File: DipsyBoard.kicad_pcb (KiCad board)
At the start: 2 copper layers, 22.9 x 50.8 mm, 31 parts, among them CON1 SDMMC_Card, P1 USB_OTG, P2 CONN_01X19, P3 CONN_01X19, P6 JTAG, SW1 SW_PUSH, U1 STM32L486Rx-LQFP64, U3 TPS56x200, U4 PUSBMxX4, X1 XTAL

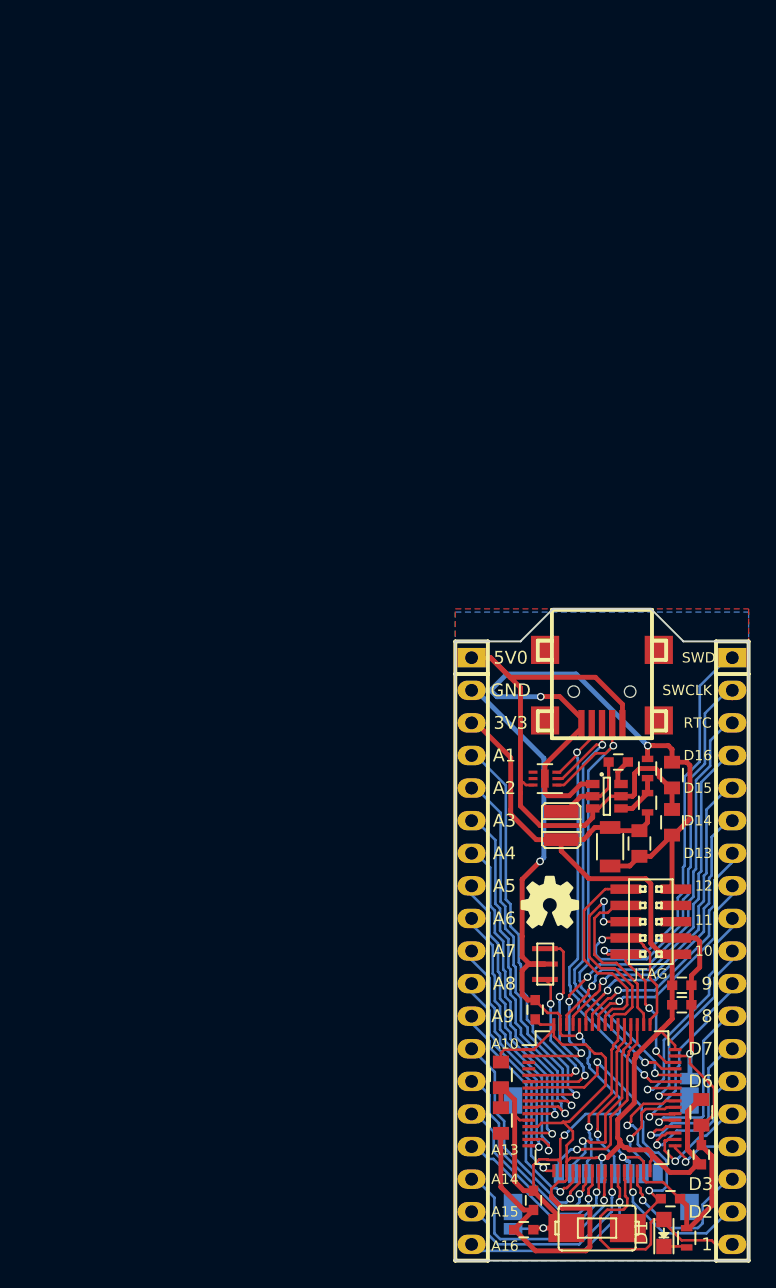
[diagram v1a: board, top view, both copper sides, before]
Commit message: v0.2
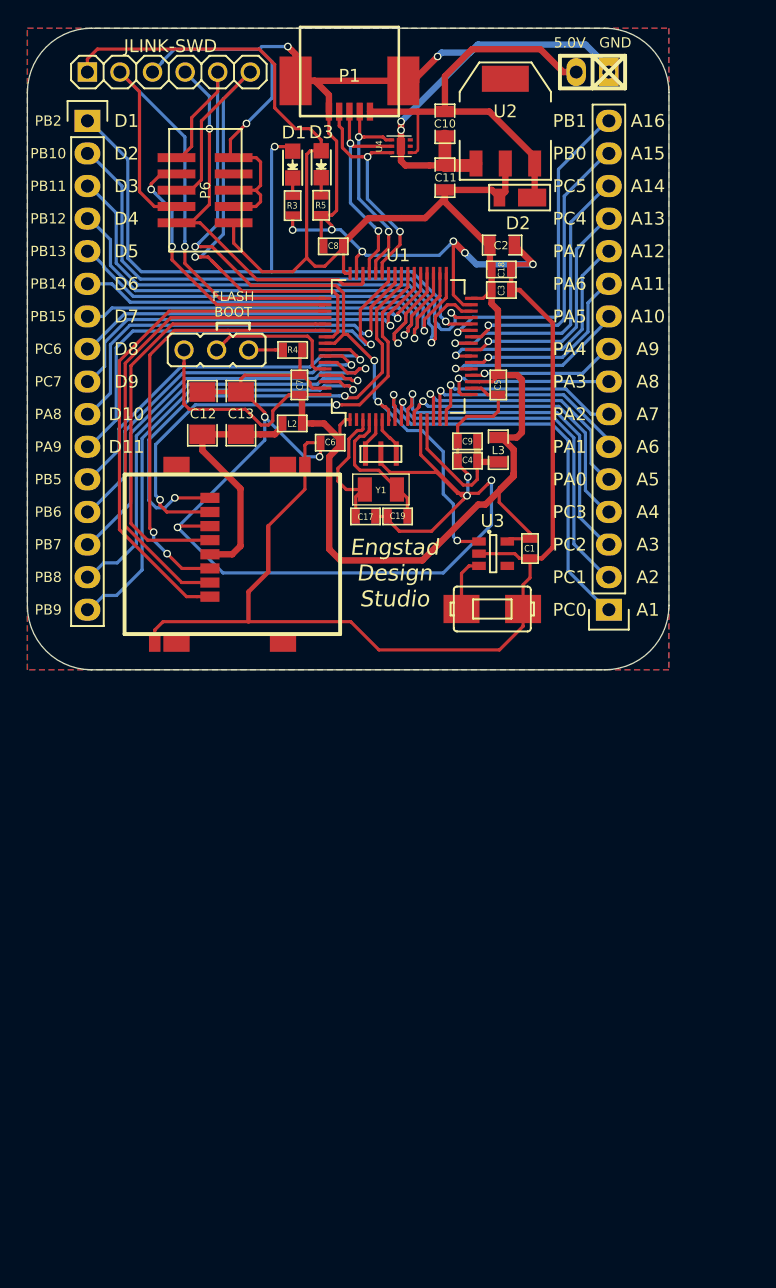
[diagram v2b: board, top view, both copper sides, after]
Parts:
- removed ?: , xess:oshw-logo2
- removed C14: 0.1uF, Capacitors_SMD:C_0603
- removed C15: 10uF, Capacitors_SMD:C_0805
- removed C16: 22uF, Capacitors_SMD:C_1206
- removed L1: 3.3uH, engstad:inductor-smd-1212
- removed R1: 33.2k, Resistors_SMD:R_0603
- removed R2: 10.0k, Resistors_SMD:R_0603
- added C12: 22uF, smd:SM1206, F.Cu at (113.6, 80.0)
- added C13: 22uF, smd:SM1206, F.Cu at (116.6, 80.0)
- added C17: 10pF, smd:SM0603, F.Cu at (126.3, 88.0)
- added C19: 10pF, smd:SM0603, F.Cu at (128.8, 88.0)
- added D2: DFLS240L, engstad:diode-smd-powerdi-123, F.Cu at (138.2, 63.2)
- added D3: GREEN, LEDs:LED-0805, F.Cu at (122.9, 60.6)
- added JP1: JUMPER3, xess:xess-JP2, F.Cu at (114.7, 75.1)
- added L2: 470nH, smd:SM0603, F.Cu at (120.6, 80.8)
- added L3: Bead, smd:SM0805, F.Cu at (136.7, 82.8)
- added P4: JLINK-SWD, xess:HDR_1x6, F.Cu at (111.0, 53.4)
- added P5: POWER, w_pin_strip:pin_socket_2, F.Cu at (144.0, 53.4)
- added R4: 10k, smd:SM0603, F.Cu at (120.7, 75.1)
- added R5: 470, smd:SM0603, F.Cu at (122.9, 63.8)
- added U2: NCP1117ST33T3G, TO_SOT_Packages_SMD:SOT-223, F.Cu at (137.2, 57.2)
- added Y1: Crystal, armory:CRYSTAL-32k-B, F.Cu at (127.5, 86.0)
- C1, C18, C5, C6, C7, C8, C9: footprint Capacitors_SMD:C_0603 -> smd:SM0603
- C10, C11, C2: footprint Capacitors_SMD:C_0805 -> smd:SM0805
- C3, C4: footprint Capacitors_SMD:C_0805 -> smd:SM0603
- CON1: footprint xess:xess-SCHD3A0100 -> engstad:SCHD3A0100; moved to F.Cu
- P1: footprint w_conn_pc:conn_usb_B_mini_smd -> engstad:usb-otg-short
- P2: value CONN_01X19 -> Analog; footprint w_pin_strip:pin_strip_19 -> Pin_Headers:Pin_Header_Straight_1x16
- P3: value CONN_01X19 -> Digital; footprint w_pin_strip:pin_strip_19 -> Pin_Headers:Pin_Header_Straight_1x16
- P6: value JTAG -> CORTEX-JTAG; footprint engstad:conn-jtag-0.05 -> engstad:smt-pin-header-02x05-127
- R3: footprint Resistors_SMD:R_0603 -> smd:SM0603
- U3: value TPS56x200 -> APX823; footprint Housings_SOT-23_SOT-143_TSOT-6:SOT-23-6 -> TO_SOT_Packages_SMD:SOT-23-5
- U4: value PUSBMxX4 -> PUSBM5V5X4; footprint Housings_DFN_QFN:DFN-6-1EP_2x2mm_Pitch0.5mm -> engstad:dfn1616-6
- moved D1 88.1 mm to (120.7, 60.6)
- moved R3 86.1 mm to (120.7, 63.8), turned to 270 degrees
- moved C18 74.9 mm to (136.9, 68.8)
- moved P3 71.3 mm to (104.7, 57.2), turned to 0 degrees
- moved C2 68.2 mm to (137.0, 66.9), turned to 0 degrees
- moved C7 67.7 mm to (121.2, 77.8)
- moved P6 66.7 mm to (113.9, 62.6)
- moved C8 63.7 mm to (123.8, 67.0), turned to 180 degrees
- moved C3 61.2 mm to (136.9, 70.4), turned to 0 degrees
- moved U1 60.7 mm to (128.9, 74.8), turned to 90 degrees
- moved C9 59.4 mm to (134.3, 82.2), turned to 180 degrees
- moved C4 54.0 mm to (134.3, 83.7), turned to 180 degrees
- moved C10 53.8 mm to (132.5, 57.4), turned to 270 degrees
- moved P1 53.7 mm to (125.1, 50.4)
- moved C11 53.3 mm to (132.5, 61.6), turned to 90 degrees
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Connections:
- net /JTDO renamed /JTDO/SWO
- C1 pad 1: /~RST -> VDD
- C11 pad 1: /OTG_5V -> VDD
- C18 pad 1: /VDD -> VDD
- C2 pad 1: /VDD -> VDD
- C3 pad 1: /VDD -> VDD
- C4 pad 1: /VDD -> +3.3VADC
- C5 pad 1: /VDD -> VDD
- C6 pad 1: /VDD -> VDD
- C7 pad 1: /VDD -> VDD
- C8 pad 1: /VDD -> VDD
- C9 pad 1: /VDD -> +3.3VADC
- CON1 pad 4: /VDD -> Net-(C12-Pad1)
- P2 pad 1: /JTMS/SWDIO -> /A1
- P2 pad 10: /D10 -> /A10
- P2 pad 11: /D9 -> /A11
- P2 pad 12: /D8 -> /A12
- P2 pad 13: /D7 -> /A13
- P2 pad 14: /D6 -> /A14
- P2 pad 15: /D5 -> /A15
- P2 pad 16: /D4 -> /A16
- P2 pad 2: /JTCK/SWCLK -> /A2
- P2 pad 3: /RTC_OUT -> /A3
- P2 pad 4: /D16 -> /A4
- P2 pad 5: /D15 -> /A5
- P2 pad 6: /D14 -> /A6
- P2 pad 7: /D13 -> /A7
- P2 pad 8: /D12 -> /A8
- P2 pad 9: /D11 -> /A9
- P3 pad 1: /OTG_5V -> /D1
- P3 pad 10: /A7 -> /D10
- P3 pad 11: /A8 -> /D11
- P3 pad 12: /A9 -> /D12
- P3 pad 13: /A10 -> /D13
- P3 pad 14: /A11 -> /D14
- P3 pad 15: /A12 -> /D15
- P3 pad 16: /A13 -> /D16
- P3 pad 2: GND -> /D2
- P3 pad 3: /VDD -> /D3
- P3 pad 4: /A1 -> /D4
- P3 pad 5: /A2 -> /D5
- P3 pad 6: /A3 -> /D6
- P3 pad 7: /A4 -> /D7
- P3 pad 8: /A5 -> /D8
- P3 pad 9: /A6 -> /D9
- P6 pad 1: /VDD -> VDD
- P6 pad 10: /~JTRST -> /~RST
- P6 pad 7: GND -> Net-(P6-Pad7)
- SW1 pad 2: /~RST -> Net-(SW1-Pad2)
- U1 pad 1: /VDD -> VDD
- U1 pad 13: /VDD -> +3.3VADC
- U1 pad 19: /VDD -> VDD
- U1 pad 2: /RTC_OUT -> /RTC
- U1 pad 3: Net-(U1-Pad3) -> /RTC_OSC_IN
- U1 pad 32: /VDD -> VDD
- U1 pad 4: Net-(U1-Pad4) -> /RTC_OSC_OUT
- U1 pad 48: /VDD -> VDD
- U1 pad 56: /~JTRST -> /~RST
- U1 pad 60: GND -> /BOOT0
- U1 pad 64: /VDD -> VDD
- U3 pad 1: GND -> /~RST
- U3 pad 2: Net-(C14-Pad1) -> GND
- U3 pad 3: /OTG_5V -> Net-(SW1-Pad2)
- U3 pad 5: /OTG_5V -> VDD
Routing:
- net VDD: track 0.00 -> 159.7 mm
- net GND: track 184.4 -> 324.1 mm, vias 8 -> 17
- net /VDD: track 136.3 -> 0.00 mm, vias 1 -> 0
- net /~RST: track 25.1 -> 64.5 mm, vias 2 -> 4
- net /RTC_OUT: track 38.0 -> 0.00 mm, vias 3 -> 0
- net /D1: track 20.6 -> 53.1 mm, vias 0 -> 2
- net /D4: track 5.74 -> 37.3 mm
- net /SDMMC_D0: track 8.32 -> 38.3 mm, vias 1 -> 2
- net /D2: track 12.0 -> 41.5 mm
- net /SDMMC_D1: track 9.76 -> 39.2 mm, vias 1 -> 2
- net /JTDO/SWO: track 16.7 -> 45.7 mm, vias 2 -> 1
- net /D3: track 12.8 -> 41.4 mm
- net /D5: track 8.76 -> 35.9 mm
- net /SDMMC_D2: track 15.7 -> 40.0 mm, vias 1 -> 0
- net /SDMMC_D3: track 14.8 -> 38.2 mm, vias 1 -> 0
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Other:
- board size 22.9 x 50.8 mm -> 50 x 50 mm
- net class Default: clearance 0.2032 -> 0.2; trace_width 0.2032 -> 0.25
- net class Power removed
- rule trace_clearance: 0.2032 -> 0.2
- rule trace_min: 0.1524 -> 0.127
- board text added: "5.0V"
- board text added: "A11"
- board text added: "A12"
- board text added: "D1"
- board text added: "D10"
- board text added: "D11"
- board text added: "D4"
- board text added: "D5"
- board text added: "D8"
- board text added: "D9"
- board text added: "FLASH BOOT"
- board text added: "PA0"
- board text added: "PA1"
- board text added: "PA2"
- board text added: "PA3"
- board text added: "PA4"
- board text added: "PA5"
- board text added: "PA6"
- board text added: "PA7"
- board text added: "PA8"
- board text added: "PA9"
- board text added: "PB0"
- board text added: "PB1"
- board text added: "PB10"
- board text added: "PB11"
- board text added: "PB12"
- board text added: "PB13"
- board text added: "PB14"
- board text added: "PB15"
- board text added: "PB2"
- board text added: "PB5"
- board text added: "PB6"
- board text added: "PB7"
- board text added: "PB8"
- board text added: "PB9"
- board text added: "PC0"
- board text added: "PC1"
- board text added: "PC2"
- board text added: "PC3"
- board text added: "PC4"
- board text added: "PC5"
- board text added: "PC6"
- board text added: "PC7"
- board text removed: "1"
- board text removed: "10"
- board text removed: "11"
- board text removed: "12"
- board text removed: "3V3"
- board text removed: "5V0"
- board text removed: "8"
- board text removed: "9"
- board text removed: "BetsyBoard V0.1"
- board text removed: "D13"
- board text removed: "D14"
- board text removed: "D15"
- board text removed: "D16"
- board text removed: "No warranty! Use at your own risk."
- board text removed: "RTC"
- board text removed: "SWCLK"
- board text removed: "SWD"
